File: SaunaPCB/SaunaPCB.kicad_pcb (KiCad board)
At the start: 2 copper layers, 199.4 x 109.2 mm, 49 parts, among them J200 KL3RM7.62, J201 KL3RM7.62, J202 KL3RM7.62, J203 KL3RM7.62, J204 KL3RM7.62, J3 KL2RM5.08, J4 KL2RM5.08, J5 KL2RM5.08, J6 KL2RM5.08, K201 Relais_SPDT_CO, K202 Relais_SPDT_CO, K203 Relais_SPDT_CO, K204 Relais_SPDT_CO, K205 Relais_SPDT_CO, K206 Relais_SPDT_CO, K207 Relais_SPDT_CO, U201 LHE05-20B24, U202 4N25, U203 4N25, U204 4N25, U4 ESP32-S3-DevKitC

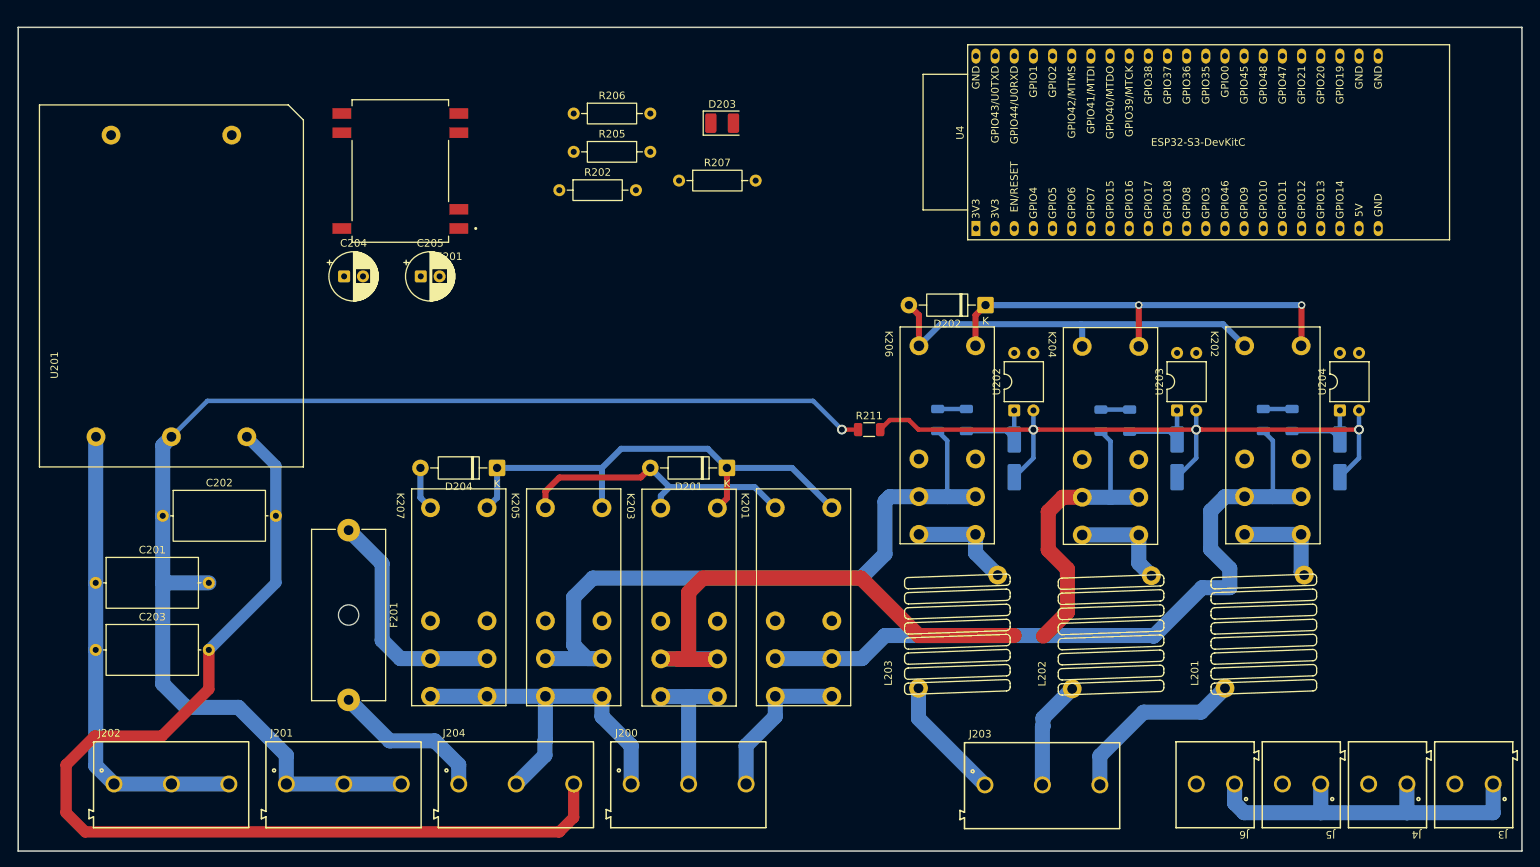
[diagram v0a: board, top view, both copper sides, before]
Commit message: Still working on placement and routing
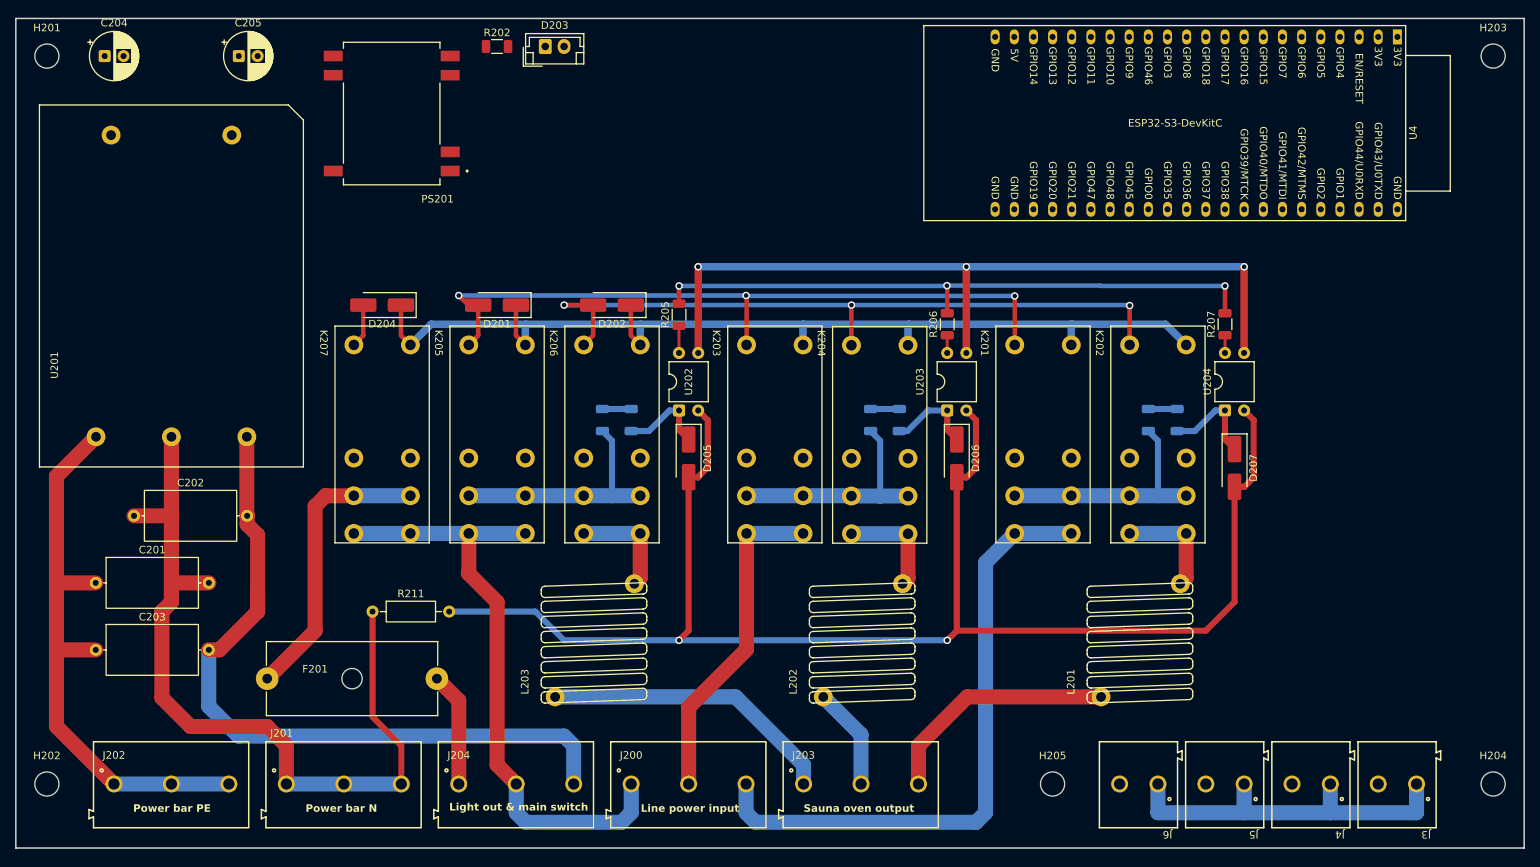
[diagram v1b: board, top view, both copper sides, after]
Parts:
- added H201: MountingHole, MountingHole:MountingHole_3.2mm_M3_DIN965, F.Cu at (71.1, 47.0)
- added H202: MountingHole, MountingHole:MountingHole_3.2mm_M3_DIN965, F.Cu at (71.1, 143.5)
- added H203: MountingHole, MountingHole:MountingHole_3.2mm_M3_DIN965, F.Cu at (262.9, 47.0)
- added H204: MountingHole, MountingHole:MountingHole_3.2mm_M3_DIN965, F.Cu at (262.9, 143.5)
- added H205: MountingHole, MountingHole:MountingHole_3.2mm_M3_DIN965, F.Cu at (204.5, 143.5)
- D201, D202, D204: footprint Diode_THT:D_DO-41_SOD81_P10.16mm_Horizontal -> Diode_SMD:D_SMA_Handsoldering
- D203: footprint LED_SMD:LED_PLCC-2_3.4x3.0mm_AK -> Connector_JST:JST_EH_B2B-EH-A_1x02_P2.50mm_Vertical
- D205, D206, D207: moved to F.Cu
- R202, R205, R206, R207: footprint Resistor_THT:R_Axial_DIN0207_L6.3mm_D2.5mm_P10.16mm_Horizontal -> Resistor_SMD:R_1206_3216Metric
- R211: footprint Resistor_SMD:R_1206_3216Metric -> Resistor_THT:R_Axial_DIN0207_L6.3mm_D2.5mm_P10.16mm_Horizontal
- moved R207 74.9 mm to (227.3, 82.5), turned to 90 degrees
- moved R211 70.1 mm to (114.3, 120.7)
- moved U4 61.4 mm to (250.2, 44.5), turned to -90 degrees
- moved R206 56.9 mm to (190.5, 82.5), turned to 90 degrees
- moved D202 49.5 mm to (146.1, 80.0)
- moved L203 48.2 mm to (143.5, 124.5)
- moved K206 44.5 mm to (146.1, 97.8)
- moved R204 44.4 mm to (148.6, 95.2)
- moved R210 44.4 mm to (144.8, 95.2)
- moved U202 44.4 mm to (154.9, 94.0)
- moved D205 43.2 mm to (156.2, 100.3)
- moved C204 43.1 mm to (78.8, 47.0)
- moved K201 38.4 mm to (203.2, 97.8)
- moved C205 37.9 mm to (96.6, 47.0)
- moved D201 37.4 mm to (130.8, 80.0)
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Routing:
- net Net-(D205-A): track 51.7 -> 200.6 mm, vias 3 -> 2
- net GND: track 48.8 -> 156.2 mm, vias 0 -> 3
- net +3V3: track 0.00 -> 82.1 mm, vias 0 -> 3
- net /Power distribution part/L2_SW: track 108.1 -> 30.6 mm
- net /Power distribution part/L1_SW: track 97.5 -> 31.8 mm
- net N: track 173.3 -> 109.0 mm, vias 1 -> 0
- net L3: track 20.7 -> 82.7 mm
- net /Power distribution part/L3_SW: track 91.7 -> 31.8 mm
- net Relais_1: track 39.4 -> 95.7 mm, vias 0 -> 3
- net L1_ON: track 141.8 -> 98.0 mm
- net Relais_2: track 54.5 -> 95.2 mm, vias 0 -> 3
- net +24V: track 102.8 -> 136.4 mm, vias 2 -> 0
- net L1: track 49.2 -> 82.5 mm
- net L2: track 19.1 -> 43.9 mm
- net /Power distribution part/L1_OUT: track 16.5 -> 39.2 mm
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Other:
- board size 199.4 x 109.2 mm -> 200 x 110 mm
- board text added: "Light out & main switch"
- board text added: "Line power input"
- board text added: "Power bar N"
- board text added: "Power bar PE"
- board text added: "Sauna oven output"
